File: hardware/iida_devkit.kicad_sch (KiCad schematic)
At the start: 7 parts

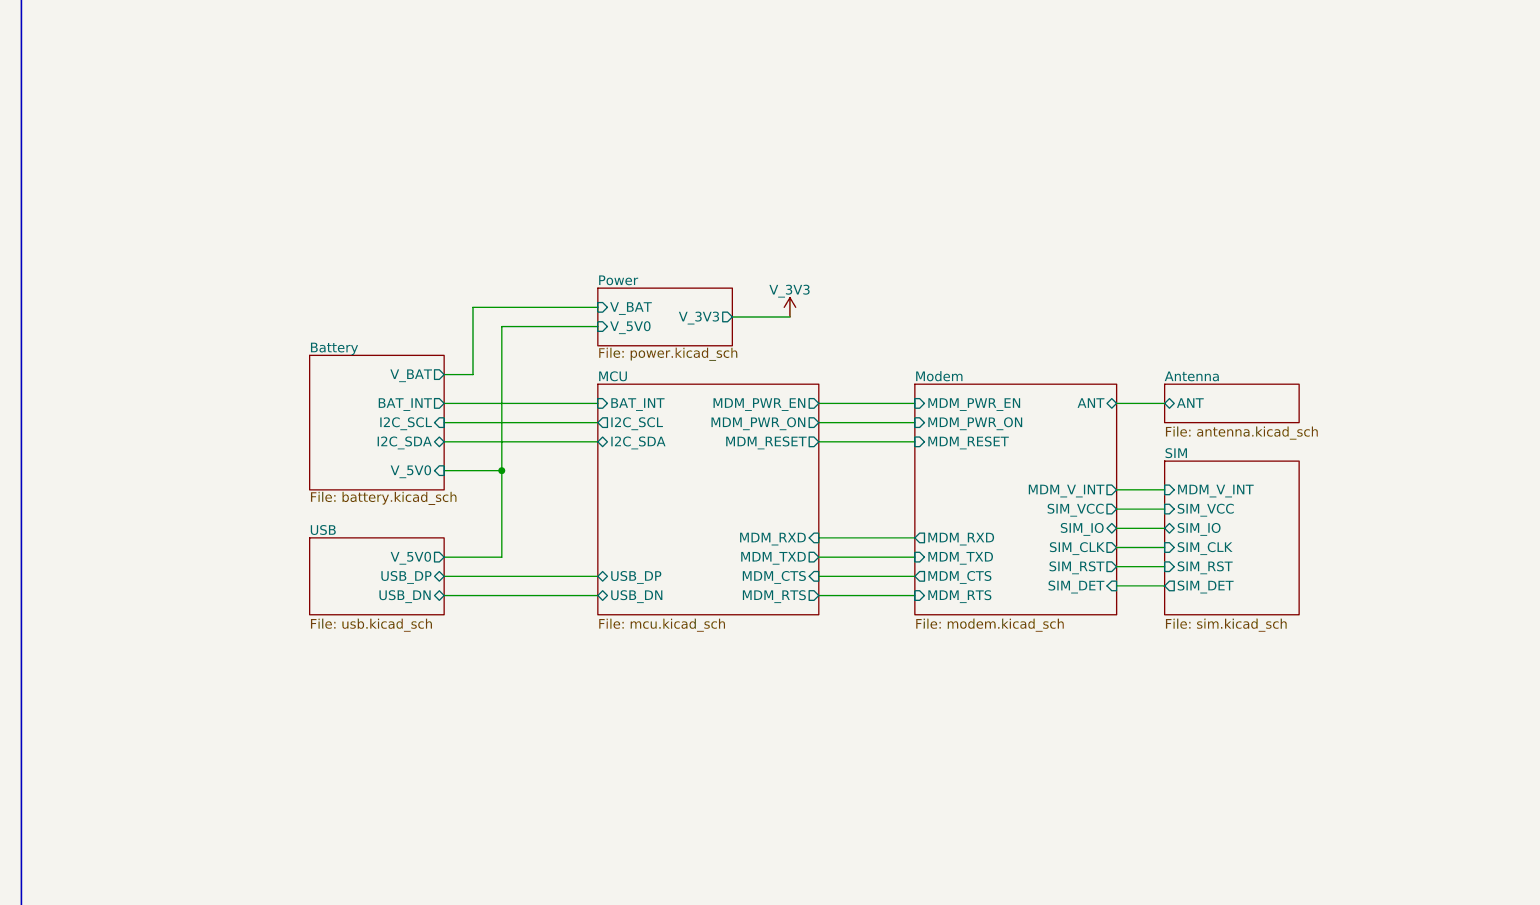
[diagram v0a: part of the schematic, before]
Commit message: HW: Reorganize schematic
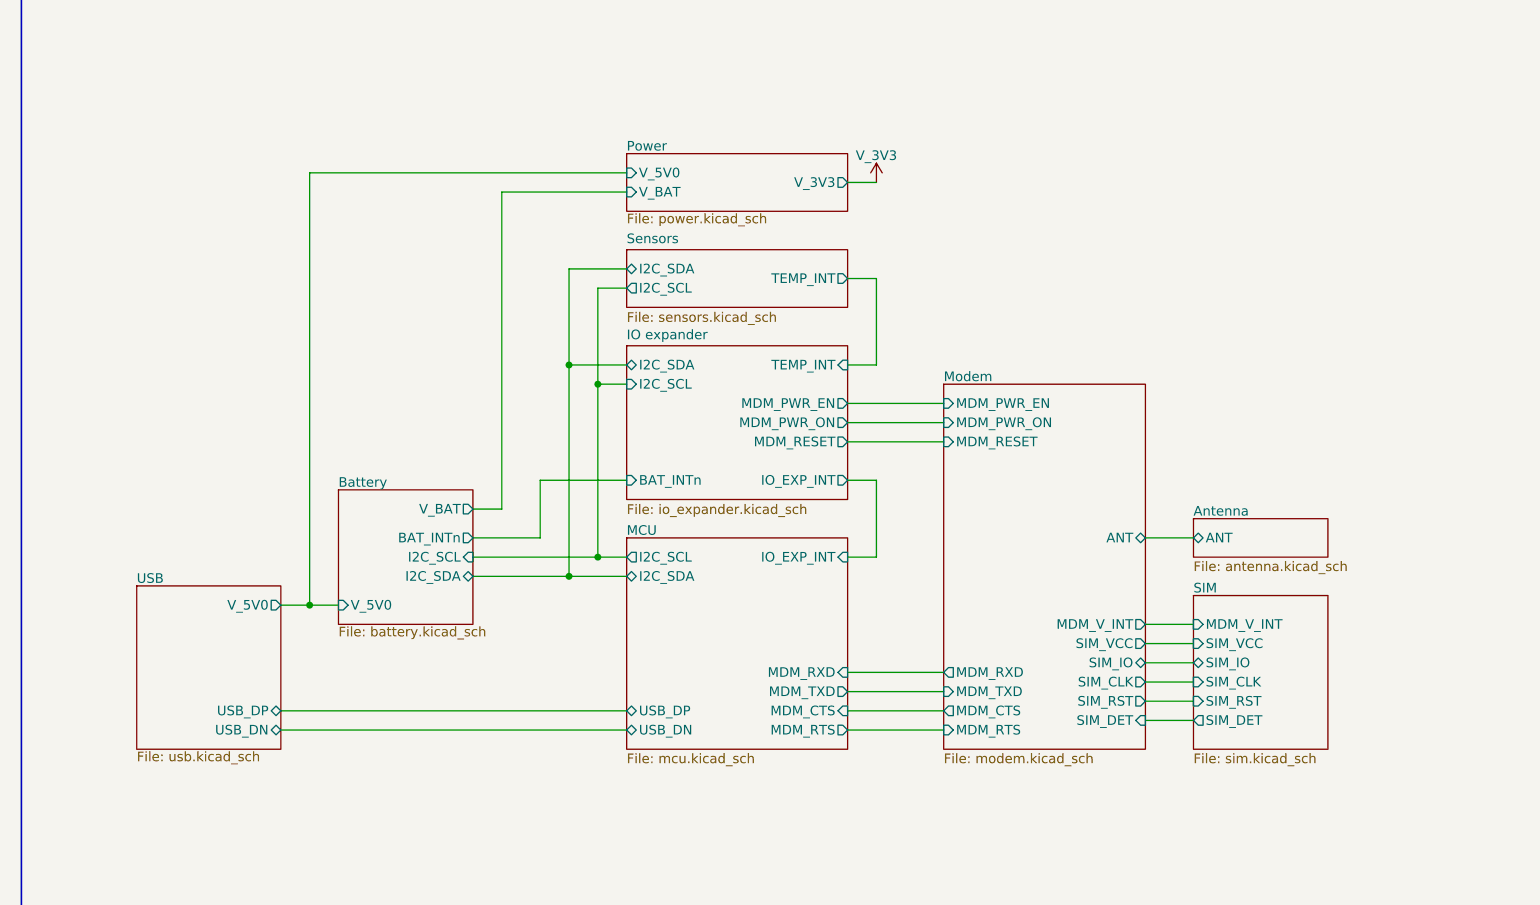
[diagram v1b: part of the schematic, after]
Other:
- added sheet IO expander (io_expander.kicad_sch)
- added sheet Sensors (sensors.kicad_sch)
- sheet Battery ports: added BAT_INTn; removed BAT_INT
- sheet MCU ports: added IO_EXP_INT; removed BAT_INT, MDM_PWR_EN, MDM_PWR_ON, MDM_RESET
